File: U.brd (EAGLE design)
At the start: 103.2 x 40 mm, 10 parts, among them IC1 LM555D, J1 1X2-3.5MM

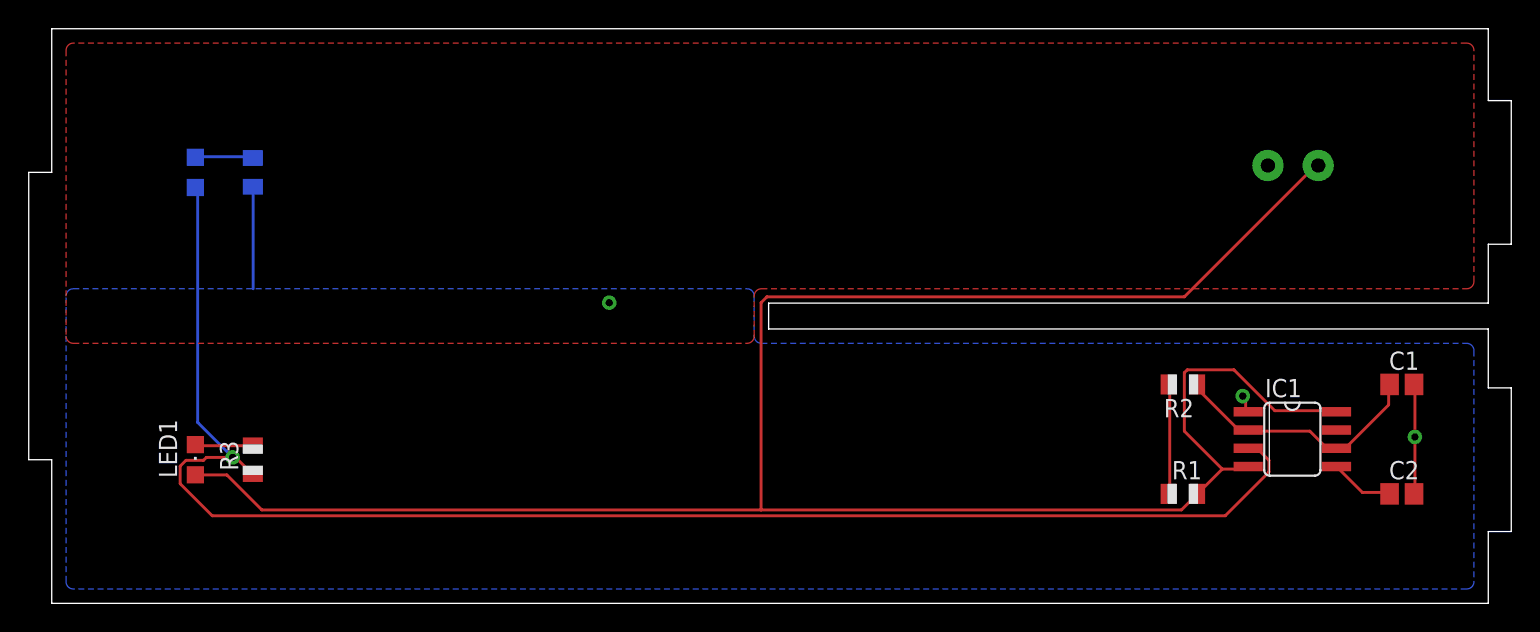
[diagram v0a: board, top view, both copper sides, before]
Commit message: reworked boards and gerber files
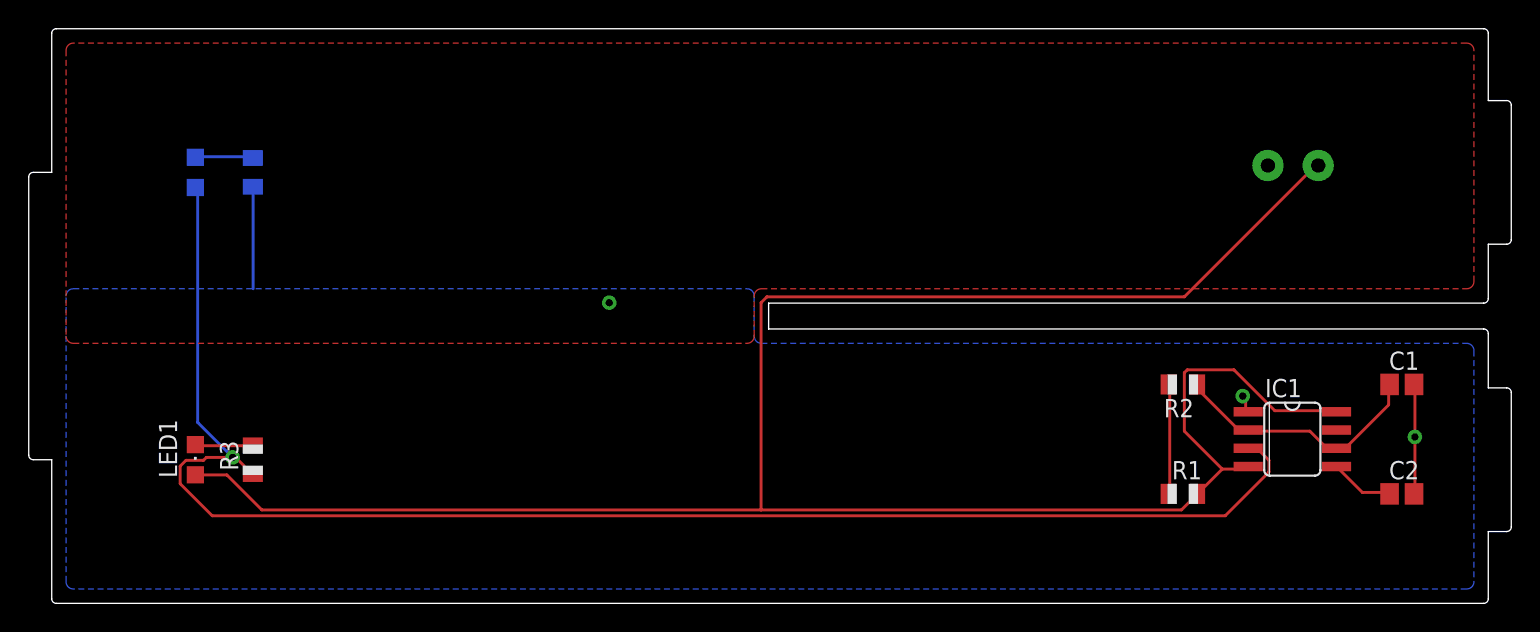
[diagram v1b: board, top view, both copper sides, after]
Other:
- outline, holes or cut-outs redrawn
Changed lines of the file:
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@@
 <layer number="45" name="Holes" color="7" fill="1" visible="no" active="yes"/>
 <layer number="46" name="Milling" color="3" fill="1" visible="no" active="yes"/>
-<layer number="47" name="Measures" color="7" fill="1" visible="no" active="yes"/>
+<layer number="47" name="Measures" color="7" fill="1" visible="yes" active="yes"/>
 <layer number="48" name="Document" color="7" fill="1" visible="no" active="yes"/>
 <layer number="49" name="Reference" color="7" fill="1" visible="no" active="yes"/>
@@
 <board>
 <plain>
-<wire x1="0" y1="10" x2="0" y2="0" width="0" layer="20"/>
-<wire x1="0" y1="0" x2="100" y2="0" width="0" layer="20"/>
-<wire x1="100" y1="0" x2="100" y2="5" width="0" layer="20"/>
-<wire x1="100" y1="5" x2="101.6" y2="5" width="0" layer="20"/>
-<wire x1="101.6" y1="5" x2="101.6" y2="15" width="0" layer="20"/>
-<wire x1="101.6" y1="15" x2="100" y2="15" width="0" layer="20"/>
-<wire x1="100" y1="15" x2="100" y2="19.1" width="0" layer="20"/>
-<wire x1="100" y1="19.1" x2="49.9" y2="19.1" width="0" layer="20"/>
+<wire x1="0" y1="10" x2="0" y2="0.3175" width="0" layer="20"/>
+<wire x1="0" y1="0.3175" x2="0.3175" y2="0" width="0" layer="20" curve="90"/>
+<wire x1="0.3175" y1="0" x2="99.6825" y2="0" width="0" layer="20"/>
+<wire x1="99.6825" y1="0" x2="100" y2="0.3175" width="0" layer="20" curve="90"/>
+<wire x1="100" y1="0.3175" x2="100" y2="5" width="0" layer="20"/>
+<wire x1="100" y1="5" x2="101.2825" y2="5" width="0" layer="20"/>
+<wire x1="101.2825" y1="5" x2="101.6" y2="5.3175" width="0" layer="20" curve="90"/>
+<wire x1="101.6" y1="5.3175" x2="101.6" y2="14.6825" width="0" layer="20"/>
+<wire x1="101.6" y1="14.6825" x2="101.2825" y2="15" width="0" layer="20" curve="90"/>
+<wire x1="101.2825" y1="15" x2="100" y2="15" width="0" layer="20"/>
+<wire x1="100" y1="15" x2="100" y2="18.7825" width="0" layer="20"/>
+<wire x1="100" y1="18.7825" x2="99.6825" y2="19.1" width="0" layer="20" curve="90"/>
+<wire x1="99.6825" y1="19.1" x2="49.9" y2="19.1" width="0" layer="20"/>
 <wire x1="49.9" y1="19.1" x2="49.9" y2="20.9" width="0" layer="20"/>
-<wire x1="49.9" y1="20.9" x2="100" y2="20.9" width="0" layer="20"/>
-<wire x1="100" y1="20.9" x2="100" y2="25" width="0" layer="20"/>
-<wire x1="100" y1="25" x2="101.6" y2="25" width="0" layer="20"/>
-<wire x1="101.6" y1="25" x2="101.6" y2="35" width="0" layer="20"/>
-<wire x1="101.6" y1="35" x2="100" y2="35" width="0" layer="20"/>
-<wire x1="100" y1="35" x2="100" y2="40" width="0" layer="20"/>
-<wire x1="100" y1="40" x2="0" y2="40" width="0" layer="20"/>
-<wire x1="0" y1="40" x2="0" y2="30" width="0" layer="20"/>
-<wire x1="0" y1="30" x2="-1.6" y2="30" width="0" layer="20"/>
-<wire x1="-1.6" y1="30" x2="-1.6" y2="10" width="0" layer="20"/>
-<wire x1="-1.6" y1="10" x2="0" y2="10" width="0" layer="20"/>
-<dimension x1="0" y1="0" x2="100" y2="0" x3="50" y3="-3.81" textsize="1.778" layer="20"/>
-<dimension x1="101.6" y1="5" x2="101.6" y2="15" x3="110" y3="10" textsize="1.778" layer="20"/>
-<dimension x1="100" y1="0" x2="100" y2="5" x3="107" y3="2.5" textsize="1.778" layer="20"/>
-<dimension x1="100" y1="15" x2="100" y2="19.1" x3="113" y3="17.05" textsize="1.778" layer="20"/>
-<dimension x1="100" y1="20.9" x2="100" y2="40" x3="104" y3="30.45" textsize="1.778" layer="20"/>
-<dimension x1="100" y1="19.1" x2="100" y2="0" x3="104" y3="9.55" textsize="1.778" layer="20"/>
-<dimension x1="0" y1="0" x2="0" y2="40" x3="-3" y3="20" textsize="1.778" layer="20"/>
-<dimension x1="-1.6" y1="30" x2="-1.6" y2="10" x3="-6" y3="20" textsize="1.778" layer="20"/>
-<dimension x1="0" y1="10" x2="0" y2="0" x3="-6" y3="5" textsize="1.778" layer="20"/>
-<dimension x1="0" y1="40" x2="0" y2="30" x3="-6" y3="35" textsize="1.778" layer="20"/>
-<dimension x1="100" y1="19.1" x2="100" y2="20.9" x3="116" y3="20" textsize="1.778" layer="20"/>
-<dimension x1="101.6" y1="35" x2="100" y2="35" x3="100.8" y3="42" textsize="1.778" layer="20"/>
-<dimension x1="0" y1="30" x2="-1.6" y2="30" x3="-0.8" y3="42" textsize="1.778" layer="20"/>
+<wire x1="49.9" y1="20.9" x2="99.6825" y2="20.9" width="0" layer="20"/>
+<wire x1="99.6825" y1="20.9" x2="100" y2="21.2175" width="0" layer="20" curve="90"/>
+<wire x1="100" y1="21.2175" x2="100" y2="25" width="0" layer="20"/>
+<wire x1="100" y1="25" x2="101.2825" y2="25" width="0" layer="20"/>
+<wire x1="101.2825" y1="25" x2="101.6" y2="25.3175" width="0" layer="20" curve="90"/>
+<wire x1="101.6" y1="25.3175" x2="101.6" y2="34.6825" width="0" layer="20"/>
+<wire x1="101.6" y1="34.6825" x2="101.2825" y2="35" width="0" layer="20" curve="90"/>
+<wire x1="101.2825" y1="35" x2="100" y2="35" width="0" layer="20"/>
+<wire x1="100" y1="35" x2="100" y2="39.6825" width="0" layer="20"/>
+<wire x1="100" y1="39.6825" x2="99.6825" y2="40" width="0" layer="20" curve="90"/>
+<wire x1="99.6825" y1="40" x2="0.3175" y2="40" width="0" layer="20"/>
+<wire x1="0.3175" y1="40" x2="0" y2="39.6825" width="0" layer="20" curve="90"/>
+<wire x1="0" y1="39.6825" x2="0" y2="30" width="0" layer="20"/>
+<wire x1="0" y1="30" x2="-1.2825" y2="30" width="0" layer="20"/>
+<wire x1="-1.2825" y1="30" x2="-1.6" y2="29.6825" width="0" layer="20" curve="90"/>
+<wire x1="-1.6" y1="29.6825" x2="-1.6" y2="10.3175" width="0" layer="20"/>
+<wire x1="-1.6" y1="10.3175" x2="-1.2825" y2="10" width="0" layer="20" curve="90"/>
+<wire x1="-1.2825" y1="10" x2="0" y2="10" width="0" layer="20"/>
+<dimension x1="0" y1="0" x2="100" y2="0" x3="50" y3="-3.81" textsize="1.778" layer="47"/>
+<dimension x1="101.6" y1="5" x2="101.6" y2="15" x3="110" y3="10" textsize="1.778" layer="47"/>
+<dimension x1="100" y1="0" x2="100" y2="5" x3="107" y3="2.5" textsize="1.778" layer="47"/>
+<dimension x1="100" y1="15" x2="100" y2="19.1" x3="113" y3="17.05" textsize="1.778" layer="47"/>
+<dimension x1="100" y1="20.9" x2="100" y2="40" x3="104" y3="30.45" textsize="1.778" layer="47"/>
+<dimension x1="100" y1="19.1" x2="100" y2="0" x3="104" y3="9.55" textsize="1.778" layer="47"/>
+<dimension x1="0" y1="0" x2="0" y2="40" x3="-3" y3="20" textsize="1.778" layer="47"/>
+<dimension x1="-1.6" y1="30" x2="-1.6" y2="10" x3="-6" y3="20" textsize="1.778" layer="47"/>
+<dimension x1="0" y1="10" x2="0" y2="0" x3="-6" y3="5" textsize="1.778" layer="47"/>
+<dimension x1="0" y1="40" x2="0" y2="30" x3="-6" y3="35" textsize="1.778" layer="47"/>
+<dimension x1="100" y1="19.1" x2="100" y2="20.9" x3="116" y3="20" textsize="1.778" layer="47"/>
+<dimension x1="101.6" y1="35" x2="100" y2="35" x3="100.8" y3="42" textsize="1.778" layer="47"/>
+<dimension x1="0" y1="30" x2="-1.6" y2="30" x3="-0.8" y3="42" textsize="1.778" layer="47"/>
 </plain>
 <attributes>
